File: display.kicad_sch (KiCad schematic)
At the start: 20 parts, among them U201 QS6K1FRATR, U202 LTP-3784E, U203 PCA9685PW

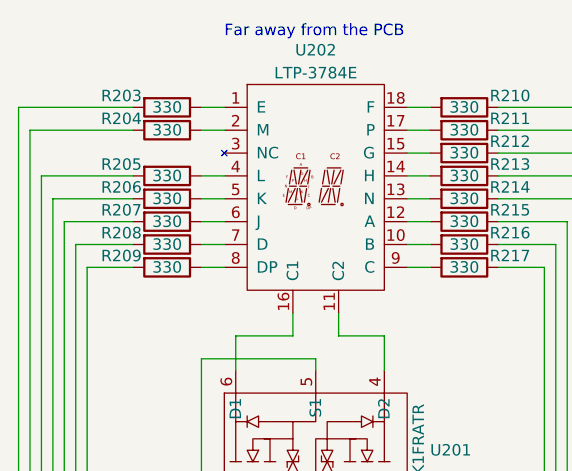
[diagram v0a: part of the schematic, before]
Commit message: finish routing(?)
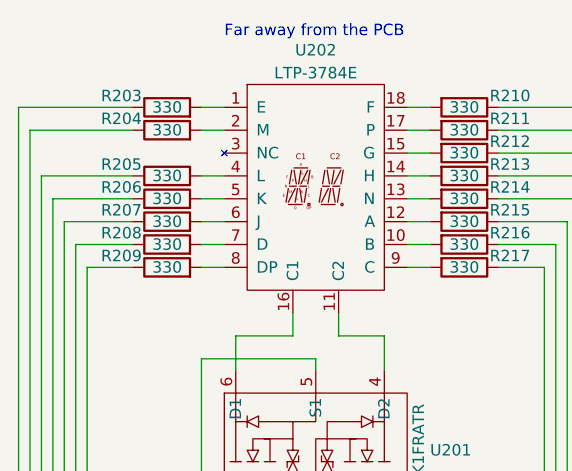
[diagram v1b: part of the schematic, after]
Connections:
- net at R206.1: now also U203.9 (LED3); no longer U202.5 (K)
- net at R206.2: now also U202.5 (K); no longer U203.9 (LED3)
- net at R203.1: now also U203.6 (LED0); no longer U202.1 (E)
- net at R203.2: now also U202.1 (E); no longer U203.6 (LED0)
- net at R207.1: now also U203.10 (LED4); no longer U202.6 (J)
- net at R207.2: now also U202.6 (J); no longer U203.10 (LED4)
- net at U203.11 (LED5): now also R208.1; no longer R208.2
- net at U203.12 (LED6): now also R209.1; no longer R209.2
- net at U203.7 (LED1): now also R204.1; no longer R204.2
- net at U203.8 (LED2): now also R205.1; no longer R205.2
- net at U202.2 (M): now also R204.2; no longer R204.1
- net at U202.4 (L): now also R205.2; no longer R205.1
- net at U202.7 (D): now also R208.2; no longer R208.1
- net at U202.8 (DP): now also R209.2; no longer R209.1
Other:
- moved on the sheet: R203, R204, R205, R206, R207, R208, R209
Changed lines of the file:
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@@
     (pin "2")
   )
-  (symbol (lib_id "Device:R") (at 111.76 45.72 270) (unit 1)
+  (symbol (lib_id "Device:R") (at 111.76 45.72 90) (unit 1)
     (in_bom yes) (on_board yes)
     (property "Reference" "R206" (id 0) (at 106.68 44.45 90))
     (property "Value" "330" (id 1) (at 111.76 45.72 90))
-    (property "Footprint" "Resistor_SMD:R_0805_2012Metric" (id 2) (at 111.76 43.942 90)
+    (property "Footprint" "Resistor_SMD:R_0805_2012Metric" (id 2) (at 111.76 47.498 90)
       (effects (font (size 1.27 1.27)) hide)
     )
@@
     (pin "2")
   )
-  (symbol (lib_id "Device:R") (at 111.76 35.56 270) (unit 1)
+  (symbol (lib_id "Device:R") (at 111.76 35.56 90) (unit 1)
     (in_bom yes) (on_board yes)
     (property "Reference" "R203" (id 0) (at 106.68 34.29 90))
     (property "Value" "330" (id 1) (at 111.76 35.56 90))
-    (property "Footprint" "Resistor_SMD:R_0805_2012Metric" (id 2) (at 111.76 33.782 90)
+    (property "Footprint" "Resistor_SMD:R_0805_2012Metric" (id 2) (at 111.76 37.338 90)
       (effects (font (size 1.27 1.27)) hide)
     )
@@
     (pin "2")
   )
-  (symbol (lib_id "Device:R") (at 111.76 48.26 270) (unit 1)
+  (symbol (lib_id "Device:R") (at 111.76 48.26 90) (unit 1)
     (in_bom yes) (on_board yes)
     (property "Reference" "R207" (id 0) (at 106.68 46.99 90))
     (property "Value" "330" (id 1) (at 111.76 48.26 90))
-    (property "Footprint" "Resistor_SMD:R_0805_2012Metric" (id 2) (at 111.76 46.482 90)
+    (property "Footprint" "Resistor_SMD:R_0805_2012Metric" (id 2) (at 111.76 50.038 90)
       (effects (font (size 1.27 1.27)) hide)
     )
@@
     (pin "6")
   )
-  (symbol (lib_id "Device:R") (at 111.76 38.1 270) (unit 1)
+  (symbol (lib_id "Device:R") (at 111.76 38.1 90) (unit 1)
     (in_bom yes) (on_board yes)
     (property "Reference" "R204" (id 0) (at 106.68 36.83 90))
     (property "Value" "330" (id 1) (at 111.76 38.1 90))
-    (property "Footprint" "Resistor_SMD:R_0805_2012Metric" (id 2) (at 111.76 36.322 90)
+    (property "Footprint" "Resistor_SMD:R_0805_2012Metric" (id 2) (at 111.76 39.878 90)
       (effects (font (size 1.27 1.27)) hide)
     )
@@
     (pin "2")
   )
-  (symbol (lib_id "Device:R") (at 111.76 43.18 270) (unit 1)
+  (symbol (lib_id "Device:R") (at 111.76 43.18 90) (unit 1)
     (in_bom yes) (on_board yes)
     (property "Reference" "R205" (id 0) (at 106.68 41.91 90))
     (property "Value" "330" (id 1) (at 111.76 43.18 90))
-    (property "Footprint" "Resistor_SMD:R_0805_2012Metric" (id 2) (at 111.76 41.402 90)
+    (property "Footprint" "Resistor_SMD:R_0805_2012Metric" (id 2) (at 111.76 44.958 90)
       (effects (font (size 1.27 1.27)) hide)
     )
@@
     (pin "2")
   )
-  (symbol (lib_id "Device:R") (at 111.76 53.34 270) (unit 1)
+  (symbol (lib_id "Device:R") (at 111.76 53.34 90) (unit 1)
     (in_bom yes) (on_board yes)
     (property "Reference" "R209" (id 0) (at 106.68 52.07 90))
     (property "Value" "330" (id 1) (at 111.76 53.34 90))
-    (property "Footprint" "Resistor_SMD:R_0805_2012Metric" (id 2) (at 111.76 51.562 90)
+    (property "Footprint" "Resistor_SMD:R_0805_2012Metric" (id 2) (at 111.76 55.118 90)
       (effects (font (size 1.27 1.27)) hide)
     )
@@
     (pin "2")
   )
-  (symbol (lib_id "Device:R") (at 111.76 50.8 270) (unit 1)
+  (symbol (lib_id "Device:R") (at 111.76 50.8 90) (unit 1)
     (in_bom yes) (on_board yes)
     (property "Reference" "R208" (id 0) (at 106.68 49.53 90))
     (property "Value" "330" (id 1) (at 111.76 50.8 90))
-    (property "Footprint" "Resistor_SMD:R_0805_2012Metric" (id 2) (at 111.76 49.022 90)
-      (effects (font (size 1.27 1.27)) hide)
-    )
+    (property "Footprint" "Resistor_SMD:R_0805_2012Metric" (id 2) (at 111.76 52.578 90)
+      (effects (font (size 1.27 1.27)) hide)
+    )
